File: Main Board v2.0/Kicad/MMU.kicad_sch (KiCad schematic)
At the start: 34 parts, among them U1 74HCT245, U2 GLT725608, U3 74HCT245, U4 GLT725608

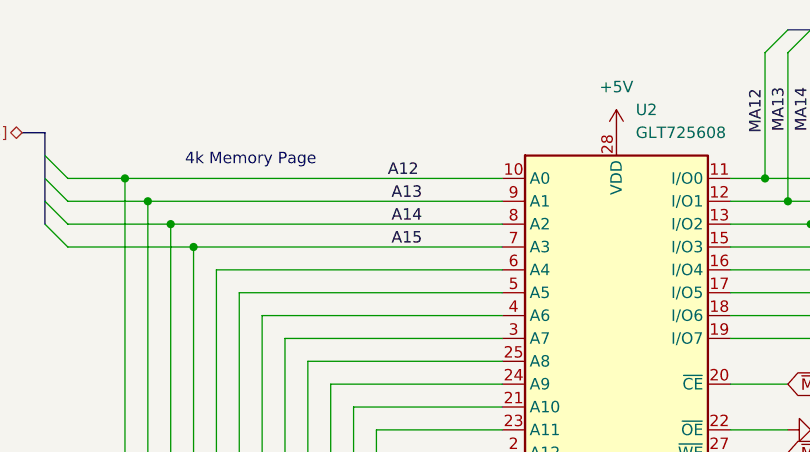
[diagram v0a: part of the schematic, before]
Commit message: board progress
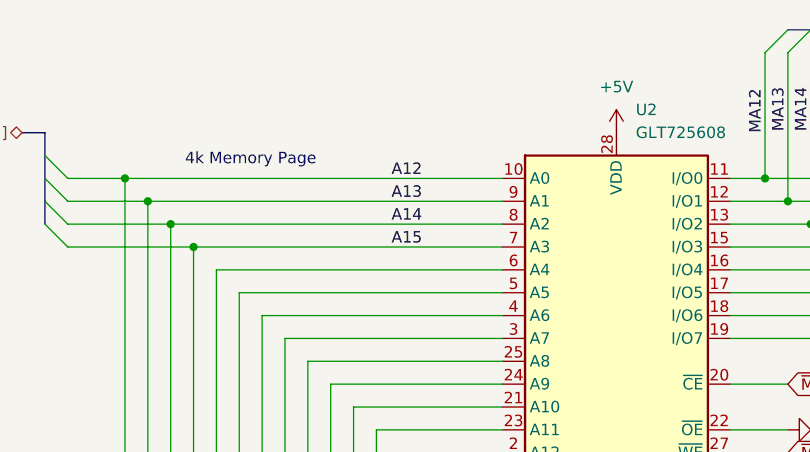
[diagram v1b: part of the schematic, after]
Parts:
- U1, U3: footprint Package_DIP:DIP-20_W7.62mm_Socket_LongPads -> Library:DIP-20_W7.62mm_Socket_LongNarrowPads
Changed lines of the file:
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@@
 	)
 	(label "A12"
-		(at 68.58 43.18 0)
+		(at 72.39 43.18 180)
 		(effects
 			(font
 				(size 1.27 1.27)
 			)
-			(justify left bottom)
+			(justify right bottom)
 		)
 	)
@@
 			)
 		)
-		(property "Footprint" "Package_DIP:DIP-20_W7.62mm_Socket_LongPads"
+		(property "Footprint" "Library:DIP-20_W7.62mm_Socket_LongNarrowPads"
 			(at 194.31 123.19 0)
 			(hide yes)
@@
 			)
 		)
-		(property "Footprint" "Package_DIP:DIP-20_W7.62mm_Socket_LongPads"
+		(property "Footprint" "Library:DIP-20_W7.62mm_Socket_LongNarrowPads"
 			(at 194.31 55.88 0)
 			(hide yes)
